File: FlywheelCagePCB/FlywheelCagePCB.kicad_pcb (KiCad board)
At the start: 2 copper layers, 43.3 x 21.2 mm, 23 parts, among them J1 Conn_01x05, J2 Conn_01x05, U1 QRE1113GR, U2 SN74LVC2G14DBV, U3 SPX3819M5-L-3-3

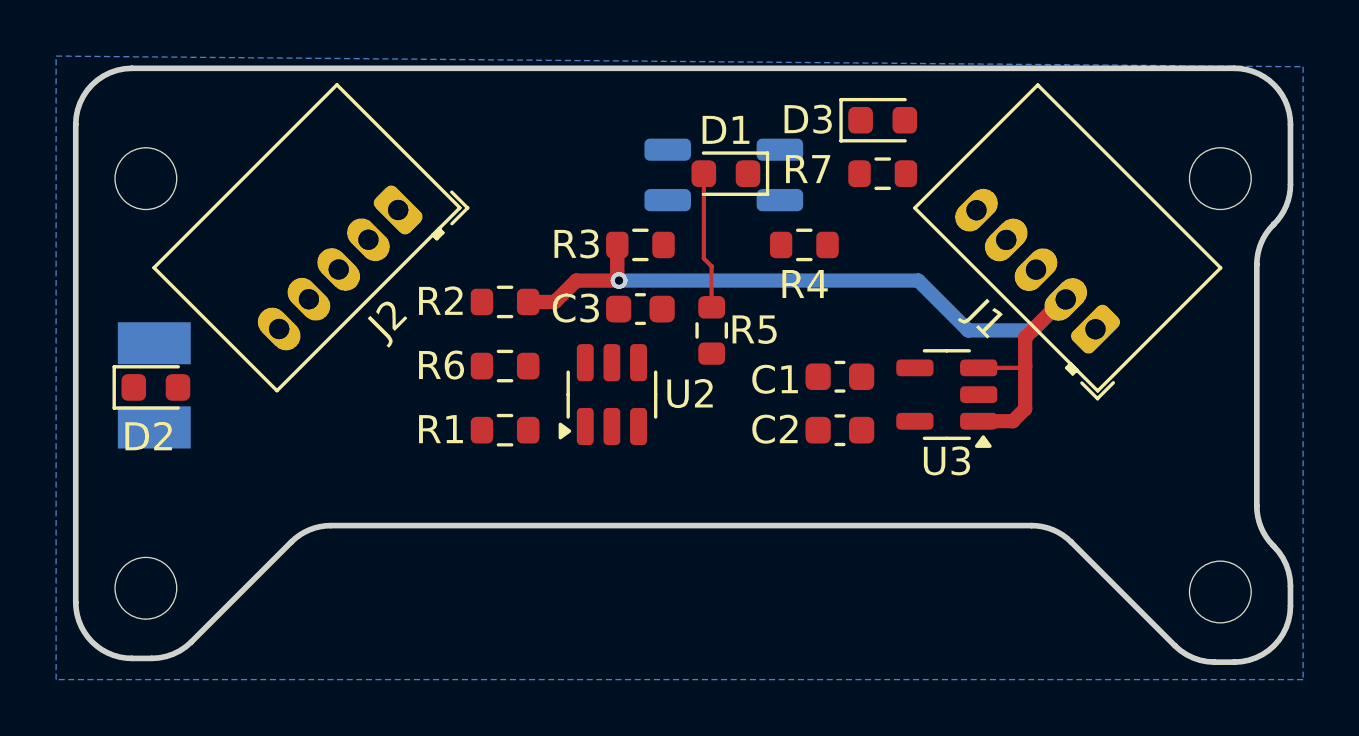
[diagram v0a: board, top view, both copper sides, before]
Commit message: Tape out on V0.1
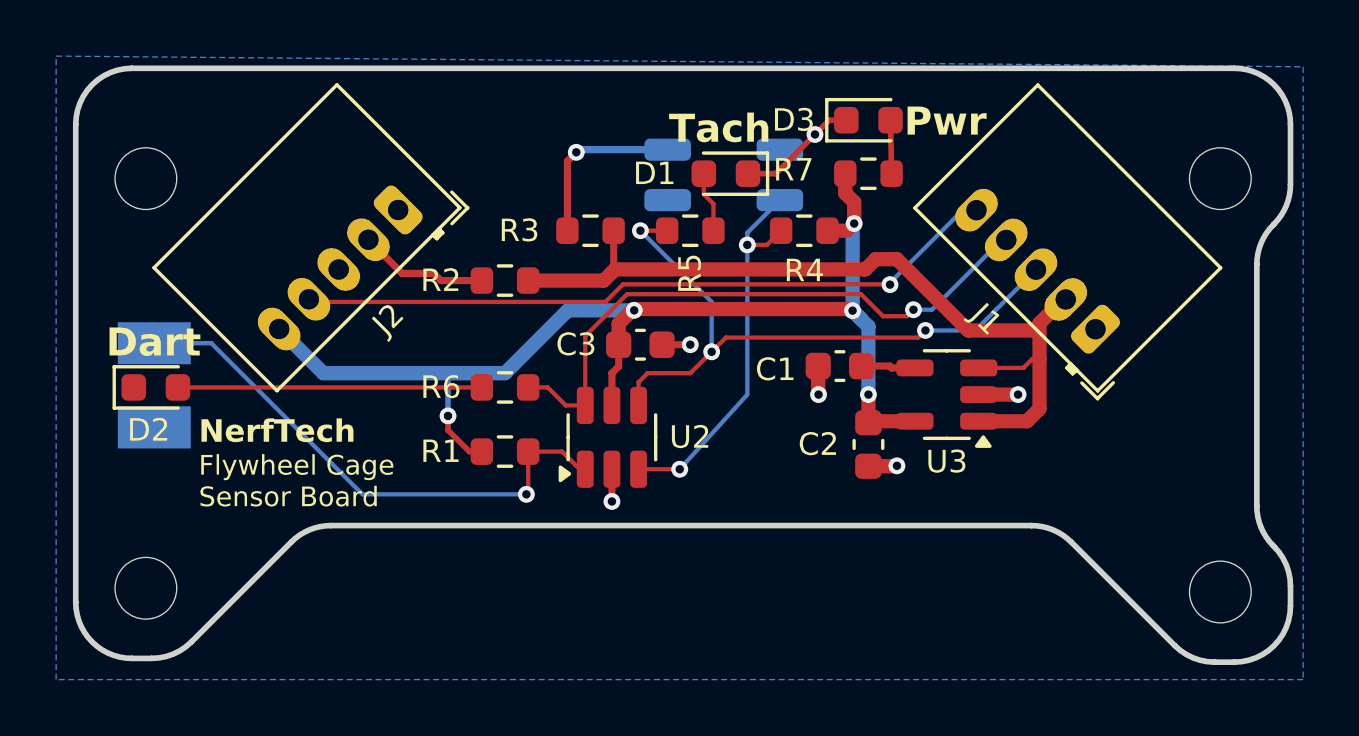
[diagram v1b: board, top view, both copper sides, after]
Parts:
- moved R5 3.64 mm to (98.8, 94.5), turned to 0 degrees
- moved R3 1.85 mm to (95.2, 94.5), turned to 180 degrees
- moved U2 1.52 mm to (96.0, 101.9)
- moved C3 1.27 mm to (97.0, 98.6)
- moved C2 1.14 mm to (105.2, 102.1), turned to -90 degrees
- moved R1 0.76 mm to (92.2, 102.4)
- moved R2 0.76 mm to (92.2, 96.3)
- moved R6 0.76 mm to (92.2, 100.1)
- moved D3 0.51 mm to (105.2, 90.6)
- moved R4 0.51 mm to (102.9, 94.5)
- moved R7 0.51 mm to (105.2, 92.5)
- moved C1 0.38 mm to (104.1, 99.3)
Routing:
- net +3.3V: track 0.00 -> 41.6 mm, vias 0 -> 5
- net temp2: track 0.00 -> 25.2 mm, vias 0 -> 1
- net /tach_d: track 0.00 -> 23.0 mm, vias 0 -> 3
- net /breakbeam_d: track 0.00 -> 21.8 mm, vias 0 -> 1
- net /breakbeam_a: track 0.00 -> 19.3 mm, vias 0 -> 1
- net /tach_a: track 0.00 -> 13.9 mm, vias 0 -> 2
- net /breakbeam_led_ind: track 0.00 -> 10.8 mm
- net GND: track 0.00 -> 9.89 mm, vias 0 -> 6
- net /tach_led: track 0.00 -> 6.22 mm, vias 0 -> 1
- net /breakbeam_led: track 0.00 -> 4.65 mm
- net /tach_led_ind: track 4.88 -> 2.17 mm
- net Net-(U3-BP): track 0.00 -> 1.92 mm
- net /power_led_ind: track 0.00 -> 1.91 mm
- net +5V: track 30.0 -> 29.9 mm, vias 1 -> 0
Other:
- board text added: "Dart"
- board text added: "Flywheel Cage Sensor Board"
- board text added: "NerfTech"
- board text added: "Pwr"
- board text added: "Tach"

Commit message: BOM scrubb
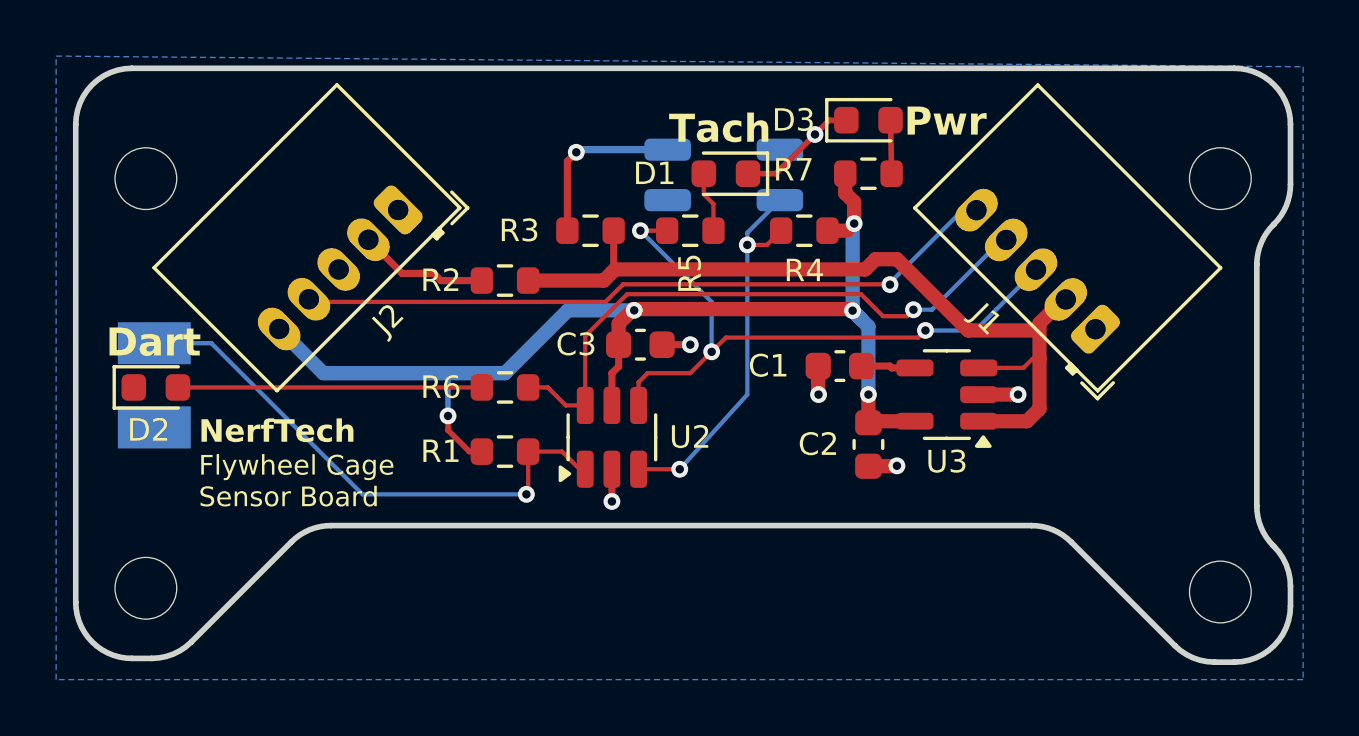
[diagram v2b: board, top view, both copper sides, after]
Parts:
- J1, J2: value Conn_01x05 -> JST_ZH_S5B
